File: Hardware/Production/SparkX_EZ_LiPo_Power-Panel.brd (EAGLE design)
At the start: 187.2 x 136.7 mm, 1656 parts, among them J10 AVR_SPI_PROG_3X2TESTPOINTS, J12 AVR_SPI_PROG_3X2TESTPOINTS, J14 AVR_SPI_PROG_3X2TESTPOINTS, J16 AVR_SPI_PROG_3X2TESTPOINTS, J18 AVR_SPI_PROG_3X2TESTPOINTS, J20 AVR_SPI_PROG_3X2TESTPOINTS, J22 AVR_SPI_PROG_3X2TESTPOINTS, J24 AVR_SPI_PROG_3X2TESTPOINTS, J26 AVR_SPI_PROG_3X2TESTPOINTS, J28 AVR_SPI_PROG_3X2TESTPOINTS, J3 AVR_SPI_PROG_3X2TESTPOINTS, J30 AVR_SPI_PROG_3X2TESTPOINTS, J32 AVR_SPI_PROG_3X2TESTPOINTS, J34 AVR_SPI_PROG_3X2TESTPOINTS, J36 AVR_SPI_PROG_3X2TESTPOINTS, J38 AVR_SPI_PROG_3X2TESTPOINTS, J4 AVR_SPI_PROG_3X2TESTPOINTS, J40 AVR_SPI_PROG_3X2TESTPOINTS, J42 AVR_SPI_PROG_3X2TESTPOINTS, J44 AVR_SPI_PROG_3X2TESTPOINTS, J46 AVR_SPI_PROG_3X2TESTPOINTS, J48 AVR_SPI_PROG_3X2TESTPOINTS, J50 AVR_SPI_PROG_3X2TESTPOINTS, J52 AVR_SPI_PROG_3X2TESTPOINTS, J54 AVR_SPI_PROG_3X2TESTPOINTS, J56 AVR_SPI_PROG_3X2TESTPOINTS, J58 AVR_SPI_PROG_3X2TESTPOINTS, J6 AVR_SPI_PROG_3X2TESTPOINTS, J60 AVR_SPI_PROG_3X2TESTPOINTS, J8 AVR_SPI_PROG_3X2TESTPOINTS, Q1 3.1A/30V/105mΩ, Q10 3.1A/30V/105mΩ, Q11 3.1A/30V/105mΩ, Q12 3.1A/30V/105mΩ, Q13 3.1A/30V/105mΩ, Q14 3.1A/30V/105mΩ, Q15 3.1A/30V/105mΩ, Q16 3.1A/30V/105mΩ, Q17 3.1A/30V/105mΩ, Q18 3.1A/30V/105mΩ, Q19 3.1A/30V/105mΩ, Q2 3.1A/30V/105mΩ, Q20 3.1A/30V/105mΩ, Q21 3.1A/30V/105mΩ, Q22 3.1A/30V/105mΩ, Q23 3.1A/30V/105mΩ, Q24 3.1A/30V/105mΩ, Q25 3.1A/30V/105mΩ, Q26 3.1A/30V/105mΩ, Q27 3.1A/30V/105mΩ, Q28 3.1A/30V/105mΩ, Q29 3.1A/30V/105mΩ, Q3 3.1A/30V/105mΩ, Q30 3.1A/30V/105mΩ, Q4 3.1A/30V/105mΩ, Q5 3.1A/30V/105mΩ, Q6 3.1A/30V/105mΩ, Q7 3.1A/30V/105mΩ, Q8 3.1A/30V/105mΩ, Q9 3.1A/30V/105mΩ, U1 STLQ015-3.3V, U10 STLQ015-3.3V, U100 STLQ015-3.3V, U101 MCP73831, U102 3.3V, U103 MAX17048, U104 ATTINY841-ARDUINO_QFN20M1, U105 STLQ015-3.3V, U106 MCP73831, U107 3.3V, U108 MAX17048, U109 ATTINY841-ARDUINO_QFN20M1, U11 MCP73831, U110 STLQ015-3.3V, U111 MCP73831, U112 3.3V, U113 MAX17048, U114 ATTINY841-ARDUINO_QFN20M1, U115 STLQ015-3.3V, U116 MCP73831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

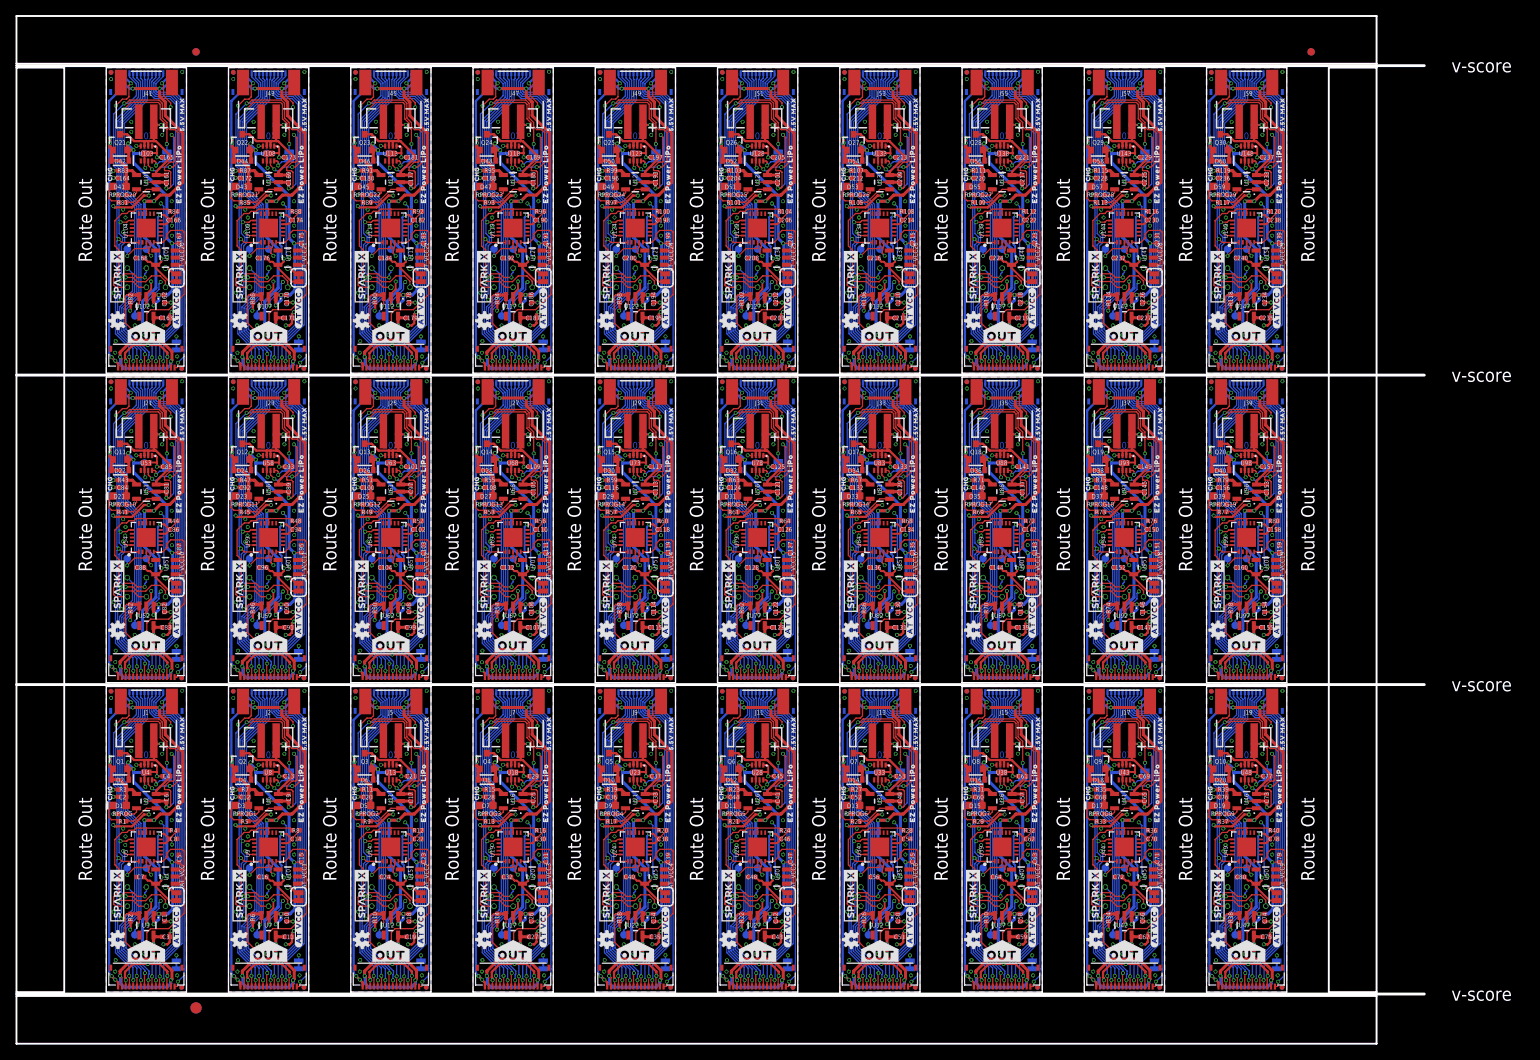
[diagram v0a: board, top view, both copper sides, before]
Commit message: Final tweaks
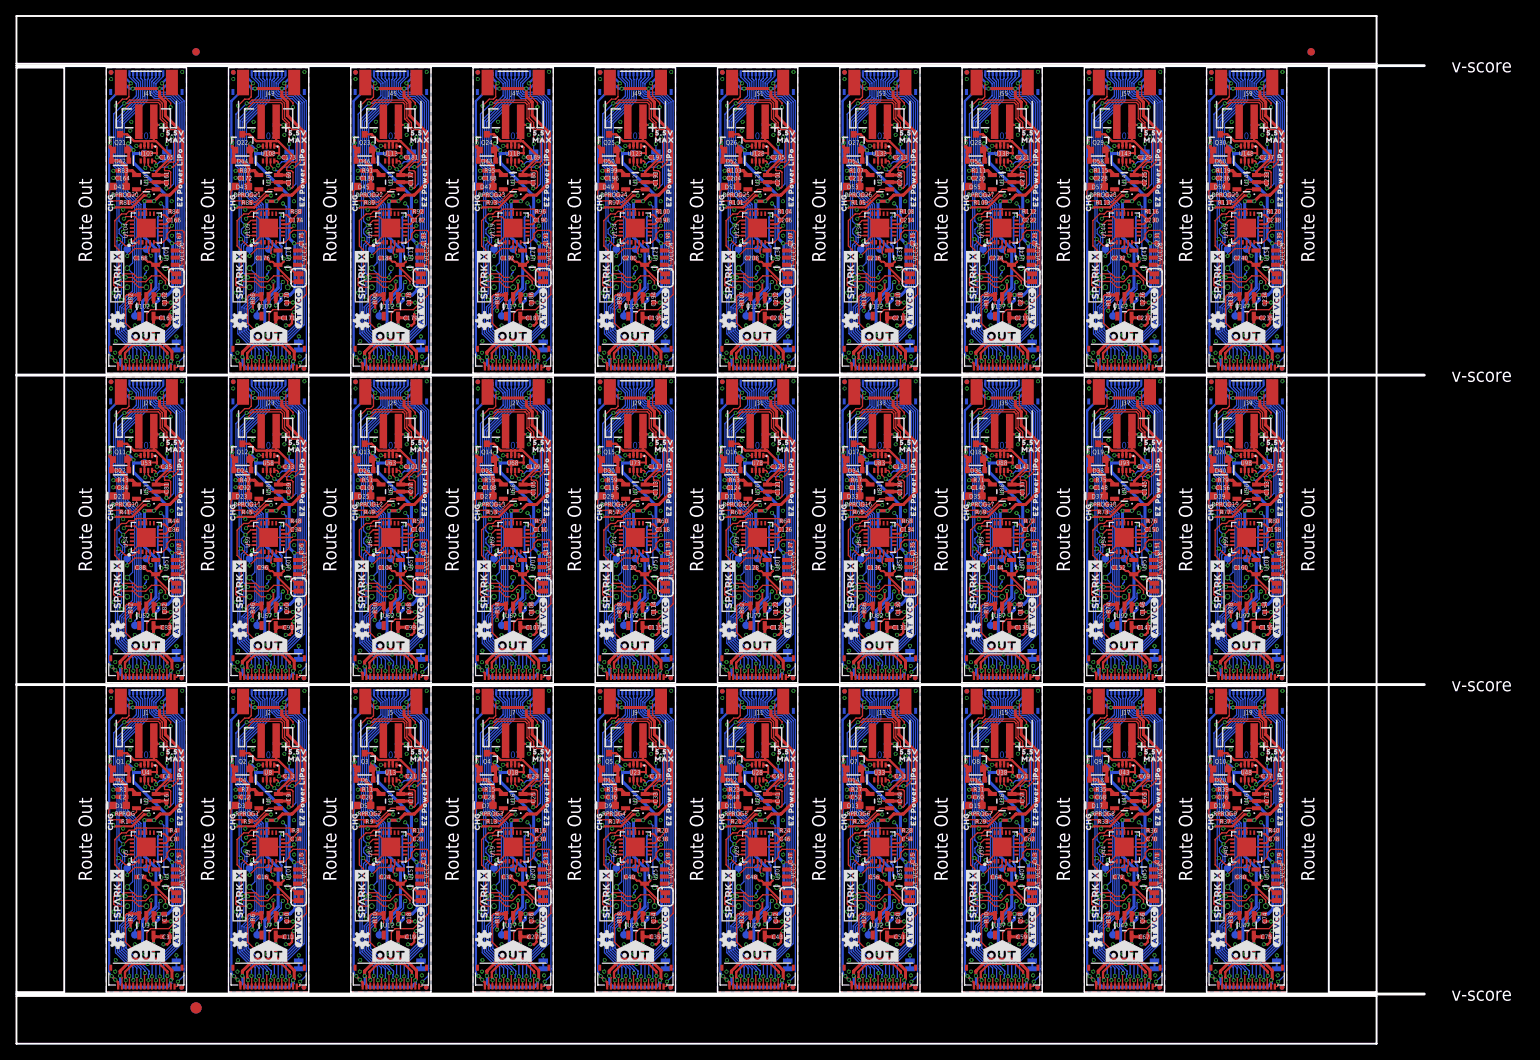
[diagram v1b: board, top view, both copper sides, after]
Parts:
- added U$481, U$482, U$498, U$499: (no value), output:EZ_POWER_LIPO0
- added U$483, U$500: (no value), output:#BATT##0
- added U$484, U$501: (no value), output:#VIN#0
- added U$485, U$502: (no value), output:#3V3_EN#0
- added U$486, U$503: (no value), output:#PROC_PWR#0
- added U$487, U$504: (no value), output:#AT_VCC#0
- added U$488, U$505: (no value), output:#FG_SDA#0
- added U$489, U$506: (no value), output:CHG0
- added U$490, U$507: (no value), output:#RXD0#0
- added U$491, U$508: (no value), output:#TXD0#0
- added U$492, U$509: (no value), output:5#5V0
- added U$493, U$510: (no value), output:MAX0
- added U$494, U$496: SPARKX-LOGO3, SparkX:SPARKX-SMALL
- added U$495: (no value), output:#OUT#0
- added U$497: (no value), output:#IN#0
- U$100, U$372: device output:#IN#0 -> output:#TXD0#0
- U$101, U$118, U$373, U$390: device output:EZ_POWER_LIPO0 -> output:5#5V0
- U$102, U$357, U$374, U$85: device output:EZ_POWER_LIPO0 -> output:MAX0
- U$103, U$343, U$375, U$71: value (none) -> SPARKX-LOGO3; device output:#BATT##0 -> SparkX:SPARKX-SMALL
- U$104, U$376: device output:#VIN#0 -> output:#OUT#0
- U$105, U$137, U$377, U$409: value (none) -> SPARKX-LOGO3; device output:#3V3_EN#0 -> SparkX:SPARKX-SMALL
- U$106, U$378: device output:#PROC_PWR#0 -> output:#IN#0
- U$107, U$363, U$379, U$91: device output:#AT_VCC#0 -> output:EZ_POWER_LIPO0
- U$108, U$124, U$380, U$396: device output:#FG_SDA#0 -> output:EZ_POWER_LIPO0
- U$109, U$381: device output:CHG0 -> output:#BATT##0
- U$11, U$238: device output:5#5V_MAX0 -> output:MAX0
- U$110, U$382: device output:5#5V_MAX0 -> output:#VIN#0
- U$111, U$383: device output:#RXD0#0 -> output:#3V3_EN#0
- U$112, U$384: device output:#TXD0#0 -> output:#PROC_PWR#0
- U$113, U$147, U$385, U$419: value SPARKX-LOGO3 -> (none); device SparkX:SPARKX-SMALL -> output:#AT_VCC#0
- U$114, U$386: device output:#OUT#0 -> output:#FG_SDA#0
- U$115, U$353, U$387, U$81: value SPARKX-LOGO3 -> (none); device SparkX:SPARKX-SMALL -> output:CHG0
- U$116, U$388: device output:#IN#0 -> output:#RXD0#0
- U$117, U$134, U$389, U$406: device output:EZ_POWER_LIPO0 -> output:#TXD0#0
- U$119, U$391: device output:#BATT##0 -> output:MAX0
- U$120, U$360, U$392, U$88: value (none) -> SPARKX-LOGO3; device output:#VIN#0 -> SparkX:SPARKX-SMALL
- U$121, U$393: device output:#3V3_EN#0 -> output:#OUT#0
- U$122, U$154, U$394, U$426: value (none) -> SPARKX-LOGO3; device output:#PROC_PWR#0 -> SparkX:SPARKX-SMALL
- U$123, U$395: device output:#AT_VCC#0 -> output:#IN#0
- U$125, U$141, U$397, U$413: device output:CHG0 -> output:EZ_POWER_LIPO0
- U$126, U$398: device output:5#5V_MAX0 -> output:#BATT##0
- U$127, U$399: device output:#RXD0#0 -> output:#VIN#0
- U$128, U$400: device output:#TXD0#0 -> output:#3V3_EN#0
- U$129, U$163, U$401, U$435: value SPARKX-LOGO3 -> (none); device SparkX:SPARKX-SMALL -> output:#PROC_PWR#0
- U$130, U$402: device output:#OUT#0 -> output:#AT_VCC#0
- U$131, U$369, U$403, U$97: value SPARKX-LOGO3 -> (none); device SparkX:SPARKX-SMALL -> output:#FG_SDA#0
- U$132, U$404: device output:#IN#0 -> output:CHG0
- U$133, U$150, U$405, U$422: device output:EZ_POWER_LIPO0 -> output:#RXD0#0
- U$135, U$407: device output:#BATT##0 -> output:5#5V0
- U$136, U$408: device output:#VIN#0 -> output:MAX0
- U$138, U$410: device output:#PROC_PWR#0 -> output:#OUT#0
- U$139, U$171, U$411, U$443: value (none) -> SPARKX-LOGO3; device output:#AT_VCC#0 -> SparkX:SPARKX-SMALL
- U$140, U$412: device output:#FG_SDA#0 -> output:#IN#0
- U$142, U$158, U$414, U$430: device output:5#5V_MAX0 -> output:EZ_POWER_LIPO0
- U$143, U$415: device output:#RXD0#0 -> output:#BATT##0
- U$144, U$416: device output:#TXD0#0 -> output:#VIN#0
- U$145, U$179, U$417, U$451: value SPARKX-LOGO3 -> (none); device SparkX:SPARKX-SMALL -> output:#3V3_EN#0
- U$146, U$418: device output:#OUT#0 -> output:#PROC_PWR#0
- U$148, U$420: device output:#IN#0 -> output:#FG_SDA#0
- U$149, U$166, U$421, U$438: device output:EZ_POWER_LIPO0 -> output:CHG0
- U$151, U$423: device output:#BATT##0 -> output:#TXD0#0
- U$152, U$424: device output:#VIN#0 -> output:5#5V0
- U$153, U$425: device output:#3V3_EN#0 -> output:MAX0
- U$155, U$427: device output:#AT_VCC#0 -> output:#OUT#0
- U$156, U$188, U$428, U$460: value (none) -> SPARKX-LOGO3; device output:#FG_SDA#0 -> SparkX:SPARKX-SMALL
- U$157, U$429: device output:CHG0 -> output:#IN#0
- U$159, U$175, U$431, U$447: device output:#RXD0#0 -> output:EZ_POWER_LIPO0
- U$16, U$305, U$33, U$339, U$67: value SPARKX-LOGO3 -> (none); device SparkX:SPARKX-SMALL -> output:5#5V0
- U$160, U$432: device output:#TXD0#0 -> output:#BATT##0
- U$161, U$195, U$433, U$467: value SPARKX-LOGO3 -> (none); device SparkX:SPARKX-SMALL -> output:#VIN#0
- U$162, U$434: device output:#OUT#0 -> output:#3V3_EN#0
- U$164, U$436: device output:#IN#0 -> output:#AT_VCC#0
- U$165, U$182, U$437, U$454: device output:EZ_POWER_LIPO0 -> output:#FG_SDA#0
- U$167, U$439: device output:#BATT##0 -> output:#RXD0#0
- U$168, U$440: device output:#VIN#0 -> output:#TXD0#0
- U$169, U$441: device output:#3V3_EN#0 -> output:5#5V0
- U$17, U$258, U$290: value (none) -> SPARKX-LOGO3; device output:#OUT#0 -> SparkX:SPARKX-SMALL
- U$170, U$442: device output:#PROC_PWR#0 -> output:MAX0
- U$172, U$444: device output:#FG_SDA#0 -> output:#OUT#0
- U$173, U$205, U$445, U$477: value (none) -> SPARKX-LOGO3; device output:CHG0 -> SparkX:SPARKX-SMALL
- U$174, U$446: device output:5#5V_MAX0 -> output:#IN#0
- U$176, U$192, U$448, U$464: device output:#TXD0#0 -> output:EZ_POWER_LIPO0
- U$177, U$211, U$449: value SPARKX-LOGO3 -> (none); device SparkX:SPARKX-SMALL -> output:#BATT##0
- U$178, U$450: device output:#OUT#0 -> output:#VIN#0
- U$18, U$257, U$291: value SPARKX-LOGO3 -> (none); device SparkX:SPARKX-SMALL -> output:#OUT#0
- U$180, U$452: device output:#IN#0 -> output:#PROC_PWR#0
- U$181, U$198, U$453, U$470: device output:EZ_POWER_LIPO0 -> output:#AT_VCC#0
- U$183, U$455: device output:#BATT##0 -> output:CHG0
- U$184, U$456: device output:#VIN#0 -> output:#RXD0#0
- U$185, U$457: device output:#3V3_EN#0 -> output:#TXD0#0
- U$186, U$458: device output:#PROC_PWR#0 -> output:5#5V0
- U$187, U$459: device output:#AT_VCC#0 -> output:MAX0
- U$189, U$461: device output:CHG0 -> output:#OUT#0
- U$19, U$292, U$324, U$52: value (none) -> SPARKX-LOGO3; device output:#IN#0 -> SparkX:SPARKX-SMALL
- U$190, U$222, U$462: value (none) -> SPARKX-LOGO3; device output:5#5V_MAX0 -> SparkX:SPARKX-SMALL
- U$191, U$463: device output:#RXD0#0 -> output:#IN#0
- U$193, U$209, U$227, U$243, U$465: value SPARKX-LOGO3 -> (none); device SparkX:SPARKX-SMALL -> output:EZ_POWER_LIPO0
- U$194, U$466: device output:#OUT#0 -> output:#BATT##0
- U$196, U$468: device output:#IN#0 -> output:#3V3_EN#0
- U$197, U$214, U$469: device output:EZ_POWER_LIPO0 -> output:#PROC_PWR#0
- U$199, U$471: device output:#BATT##0 -> output:#FG_SDA#0
- U$200, U$472: device output:#VIN#0 -> output:CHG0
- U$201, U$473: device output:#3V3_EN#0 -> output:#RXD0#0
- U$202, U$474: device output:#PROC_PWR#0 -> output:#TXD0#0
- U$203, U$475: device output:#AT_VCC#0 -> output:5#5V0
- U$204, U$476: device output:#FG_SDA#0 -> output:MAX0
- U$206, U$478: device output:5#5V_MAX0 -> output:#OUT#0
- U$207, U$239, U$479: value (none) -> SPARKX-LOGO3; device output:#RXD0#0 -> SparkX:SPARKX-SMALL
- U$208, U$480: device output:#TXD0#0 -> output:#IN#0
- U$21, U$293, U$310, U$38: device output:EZ_POWER_LIPO0 -> output:#IN#0
- U$210, U$226: device output:#OUT#0 -> output:EZ_POWER_LIPO0
- U$212: device output:#IN#0 -> output:#VIN#0
- U$213, U$230: device output:EZ_POWER_LIPO0 -> output:#3V3_EN#0
- U$215: device output:#BATT##0 -> output:#AT_VCC#0
- U$216: device output:#VIN#0 -> output:#FG_SDA#0
- U$217: device output:#3V3_EN#0 -> output:CHG0
- U$218: device output:#PROC_PWR#0 -> output:#RXD0#0
- U$219: device output:#AT_VCC#0 -> output:#TXD0#0
- U$220: device output:#FG_SDA#0 -> output:5#5V0
- U$221: device output:CHG0 -> output:MAX0
- U$223: device output:#RXD0#0 -> output:#OUT#0
- U$224, U$256: value (none) -> SPARKX-LOGO3; device output:#TXD0#0 -> SparkX:SPARKX-SMALL
- U$225, U$259: value SPARKX-LOGO3 -> (none); device SparkX:SPARKX-SMALL -> output:#IN#0
- U$228: device output:#IN#0 -> output:#BATT##0
- U$229, U$246: device output:EZ_POWER_LIPO0 -> output:#VIN#0
- U$23, U$295, U$311, U$39: device output:#BATT##0 -> output:EZ_POWER_LIPO0
- U$231: device output:#BATT##0 -> output:#PROC_PWR#0
- U$232: device output:#VIN#0 -> output:#AT_VCC#0
- U$233: device output:#3V3_EN#0 -> output:#FG_SDA#0
- U$234: device output:#PROC_PWR#0 -> output:CHG0
- U$235: device output:#AT_VCC#0 -> output:#RXD0#0
- U$236: device output:#FG_SDA#0 -> output:#TXD0#0
- U$237: device output:CHG0 -> output:5#5V0
- U$24, U$296: device output:#VIN#0 -> output:#BATT##0
- U$240: device output:#TXD0#0 -> output:#OUT#0
- U$242: device output:#OUT#0 -> output:#IN#0
- U$244, U$260: device output:#IN#0 -> output:EZ_POWER_LIPO0
- U$245, U$262: device output:EZ_POWER_LIPO0 -> output:#BATT##0
- U$247: device output:#BATT##0 -> output:#3V3_EN#0
- U$248: device output:#VIN#0 -> output:#PROC_PWR#0
- U$249: device output:#3V3_EN#0 -> output:#AT_VCC#0
- U$25, U$297: device output:#3V3_EN#0 -> output:#VIN#0
- U$250: device output:#PROC_PWR#0 -> output:#FG_SDA#0
- U$251: device output:#AT_VCC#0 -> output:CHG0
- U$252: device output:#FG_SDA#0 -> output:#RXD0#0
- U$253: device output:CHG0 -> output:#TXD0#0
- U$254: device output:5#5V_MAX0 -> output:5#5V0
- U$255: device output:#RXD0#0 -> output:MAX0
- U$26, U$298: device output:#PROC_PWR#0 -> output:#3V3_EN#0
- U$263: device output:#BATT##0 -> output:#VIN#0
- U$264: device output:#VIN#0 -> output:#3V3_EN#0
- U$265: device output:#3V3_EN#0 -> output:#PROC_PWR#0
- U$266: device output:#PROC_PWR#0 -> output:#AT_VCC#0
- U$267: device output:#AT_VCC#0 -> output:#FG_SDA#0
- U$268: device output:#FG_SDA#0 -> output:CHG0
- U$269: device output:CHG0 -> output:#RXD0#0
- U$27, U$299: device output:#AT_VCC#0 -> output:#PROC_PWR#0
- U$270: device output:5#5V_MAX0 -> output:#TXD0#0
- U$271: device output:#RXD0#0 -> output:5#5V0
- U$272: device output:#TXD0#0 -> output:MAX0
- U$28, U$300: device output:#FG_SDA#0 -> output:#AT_VCC#0
- U$286: device output:5#5V_MAX0 -> output:#RXD0#0
- U$287: device output:#RXD0#0 -> output:#TXD0#0
- U$288: device output:#TXD0#0 -> output:5#5V0
- U$289, U$323, U$51: value SPARKX-LOGO3 -> (none); device SparkX:SPARKX-SMALL -> output:MAX0
- U$29, U$301: device output:CHG0 -> output:#FG_SDA#0
- U$30, U$302: device output:5#5V_MAX0 -> output:CHG0
- U$306, U$34: device output:#OUT#0 -> output:MAX0
- U$308, U$36: device output:#IN#0 -> output:#OUT#0
- U$309, U$326, U$341, U$358, U$37, U$54, U$69, U$86: value (none) -> SPARKX-LOGO3; device output:EZ_POWER_LIPO0 -> SparkX:SPARKX-SMALL
- U$312, U$328, U$40, U$56: device output:#VIN#0 -> output:EZ_POWER_LIPO0
- U$313, U$41: device output:#3V3_EN#0 -> output:#BATT##0
- U$314, U$42: device output:#PROC_PWR#0 -> output:#VIN#0
- U$315, U$43: device output:#AT_VCC#0 -> output:#3V3_EN#0
- U$316, U$44: device output:#FG_SDA#0 -> output:#PROC_PWR#0
- U$317, U$45: device output:CHG0 -> output:#AT_VCC#0
- U$318, U$46: device output:5#5V_MAX0 -> output:#FG_SDA#0
- U$319, U$47: device output:#RXD0#0 -> output:CHG0
- U$320, U$48: device output:#TXD0#0 -> output:#RXD0#0
- U$321, U$355, U$49, U$83: value SPARKX-LOGO3 -> (none); device SparkX:SPARKX-SMALL -> output:#TXD0#0
- U$322, U$50: device output:#OUT#0 -> output:5#5V0
- U$325, U$342, U$53, U$70: device output:EZ_POWER_LIPO0 -> output:#OUT#0
- U$327, U$55: device output:#BATT##0 -> output:#IN#0
- U$329, U$345, U$57, U$73: device output:#3V3_EN#0 -> output:EZ_POWER_LIPO0
- U$330, U$58: device output:#PROC_PWR#0 -> output:#BATT##0
- U$331, U$59: device output:#AT_VCC#0 -> output:#VIN#0
- U$332, U$60: device output:#FG_SDA#0 -> output:#3V3_EN#0
- U$333, U$61: device output:CHG0 -> output:#PROC_PWR#0
- U$334, U$62: device output:5#5V_MAX0 -> output:#AT_VCC#0
- U$335, U$63: device output:#RXD0#0 -> output:#FG_SDA#0
- U$336, U$64: device output:#TXD0#0 -> output:CHG0
- U$337, U$371, U$65, U$99: value SPARKX-LOGO3 -> (none); device SparkX:SPARKX-SMALL -> output:#RXD0#0
- U$338, U$66: device output:#OUT#0 -> output:#TXD0#0
- U$340, U$68: device output:#IN#0 -> output:MAX0
- U$344, U$72: device output:#VIN#0 -> output:#IN#0
- U$346, U$362, U$74, U$90: device output:#PROC_PWR#0 -> output:EZ_POWER_LIPO0
- U$347, U$75: device output:#AT_VCC#0 -> output:#BATT##0
- U$348, U$76: device output:#FG_SDA#0 -> output:#VIN#0
- U$349, U$77: device output:CHG0 -> output:#3V3_EN#0
- U$350, U$78: device output:5#5V_MAX0 -> output:#PROC_PWR#0
- U$351, U$79: device output:#RXD0#0 -> output:#AT_VCC#0
- U$352, U$80: device output:#TXD0#0 -> output:#FG_SDA#0
- U$354, U$82: device output:#OUT#0 -> output:#RXD0#0
- U$356, U$84: device output:#IN#0 -> output:5#5V0
- U$359, U$87: device output:#BATT##0 -> output:#OUT#0
- U$361, U$89: device output:#3V3_EN#0 -> output:#IN#0
- U$364, U$92: device output:#FG_SDA#0 -> output:#BATT##0
- U$365, U$93: device output:CHG0 -> output:#VIN#0
- U$366, U$94: device output:5#5V_MAX0 -> output:#3V3_EN#0
- U$367, U$95: device output:#RXD0#0 -> output:#PROC_PWR#0
- U$368, U$96: device output:#TXD0#0 -> output:#AT_VCC#0
- U$370, U$98: device output:#OUT#0 -> output:CHG0
- moved U$164 164.7 mm to (155.6, 8.64), flipped to the top, turned to 90 degrees
- moved U$333 163.2 mm to (150.7, 44.9), flipped to the bottom, turned to 0 degrees
- moved U$168 160.8 mm to (154.4, 16.5)
- moved U$334 160.2 mm to (155.6, 49.8)
- moved U$328 159.4 mm to (156.1, 67.2), flipped to the top, turned to 90 degrees
- moved U$163 158.4 mm to (150.7, 3.75)
- moved U$335 157.2 mm to (156.1, 69.8)
- moved U$332 156.4 mm to (153.3, 48.8), turned to 0 degrees
- moved U$324 155.8 mm to (147.8, 54.0), flipped to the top, turned to 90 degrees
- moved U$167 155.7 mm to (147.9, 16.5), turned to 90 degrees
- moved U$325 155.2 mm to (151.6, 46.0), turned to 0 degrees
- moved U$327 153.5 mm to (151.6, 75.9)
- moved U$162 152.9 mm to (153.3, 7.62), flipped to the bottom
- moved U$170 151.7 mm to (155.5, 31.0), flipped to the top
- moved U$165 151.5 mm to (156.1, 28.7), flipped to the bottom
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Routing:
- net GND1: track 82.0 -> 96.0 mm
- net GND7: track 82.0 -> 96.0 mm
- net GND6: track 82.0 -> 96.0 mm
- net GND5: track 82.0 -> 96.0 mm
- net GND2: track 82.0 -> 96.0 mm
- net GND3: track 82.0 -> 96.0 mm
- net GND9: track 82.0 -> 96.0 mm
- net GND8: track 82.0 -> 96.0 mm
- net GND4: track 82.0 -> 96.0 mm
- net GND19: track 82.0 -> 96.0 mm
- net GND18: track 82.0 -> 96.0 mm
- net GND: track 82.0 -> 96.0 mm
- net GND29: track 82.0 -> 96.0 mm
- net GND28: track 82.0 -> 96.0 mm
- net GND27: track 82.0 -> 96.0 mm
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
